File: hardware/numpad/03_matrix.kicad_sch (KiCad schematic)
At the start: 36 parts, among them SW3 RotaryEncoder_Switch

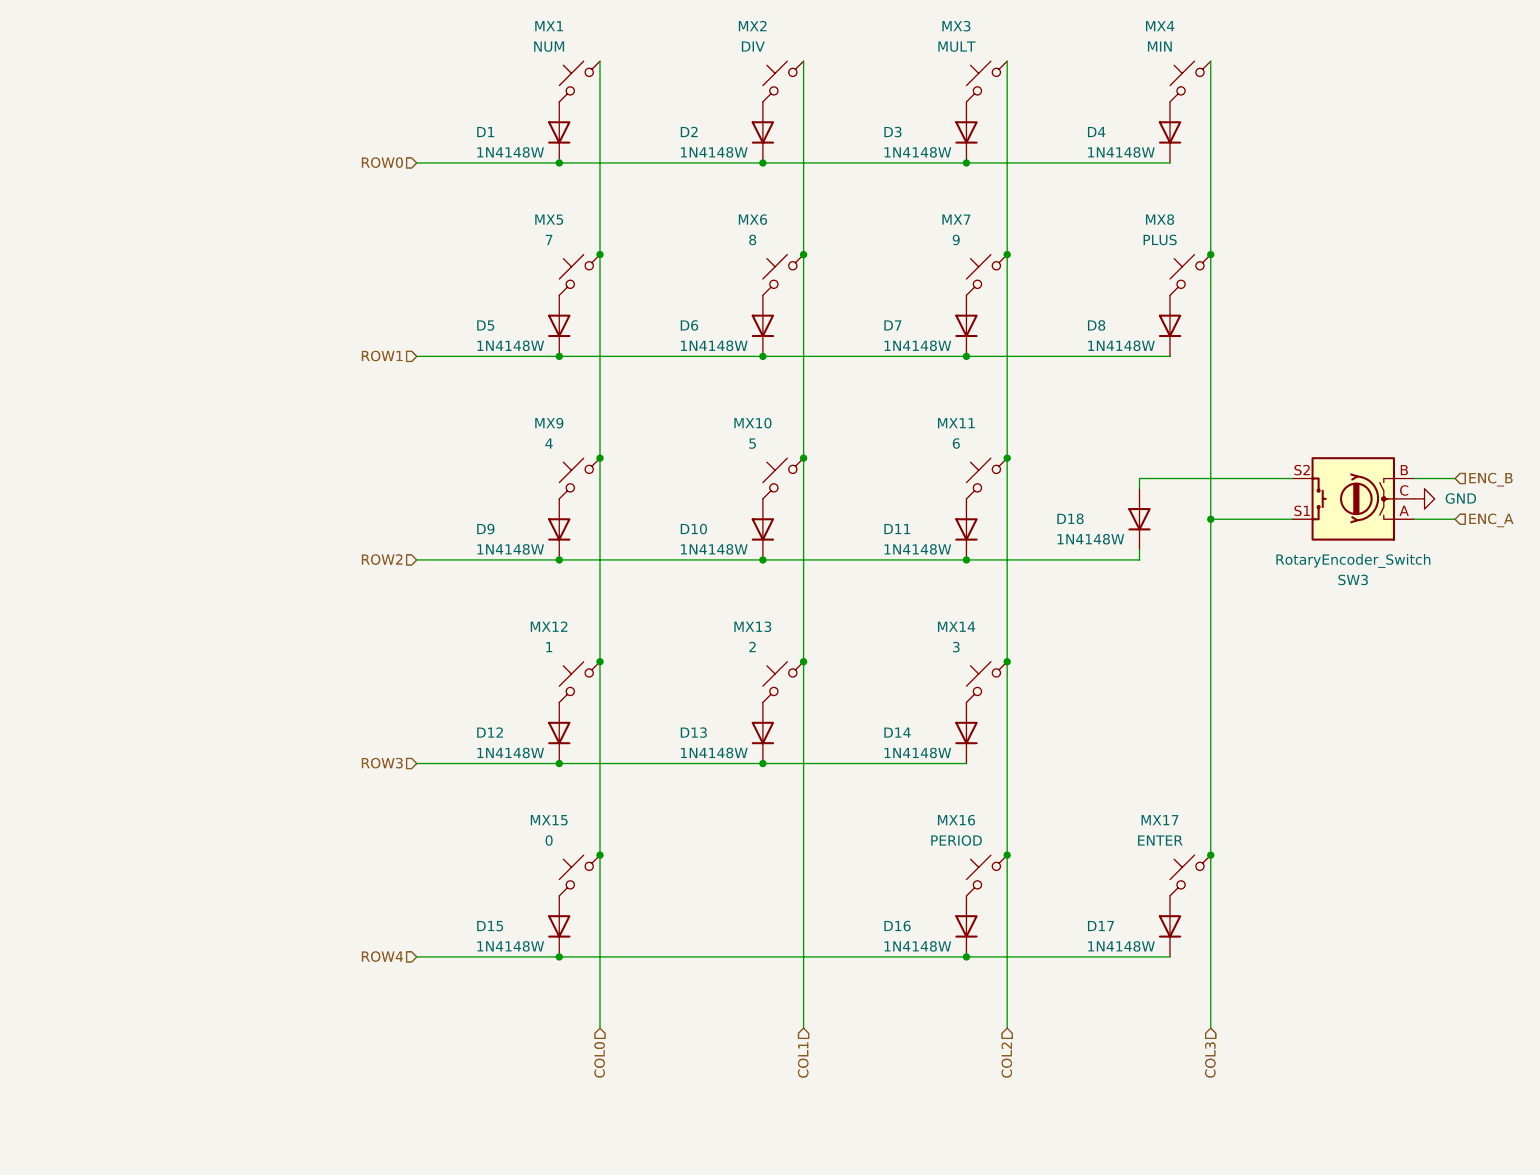
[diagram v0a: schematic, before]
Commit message: Format cleanup, titles
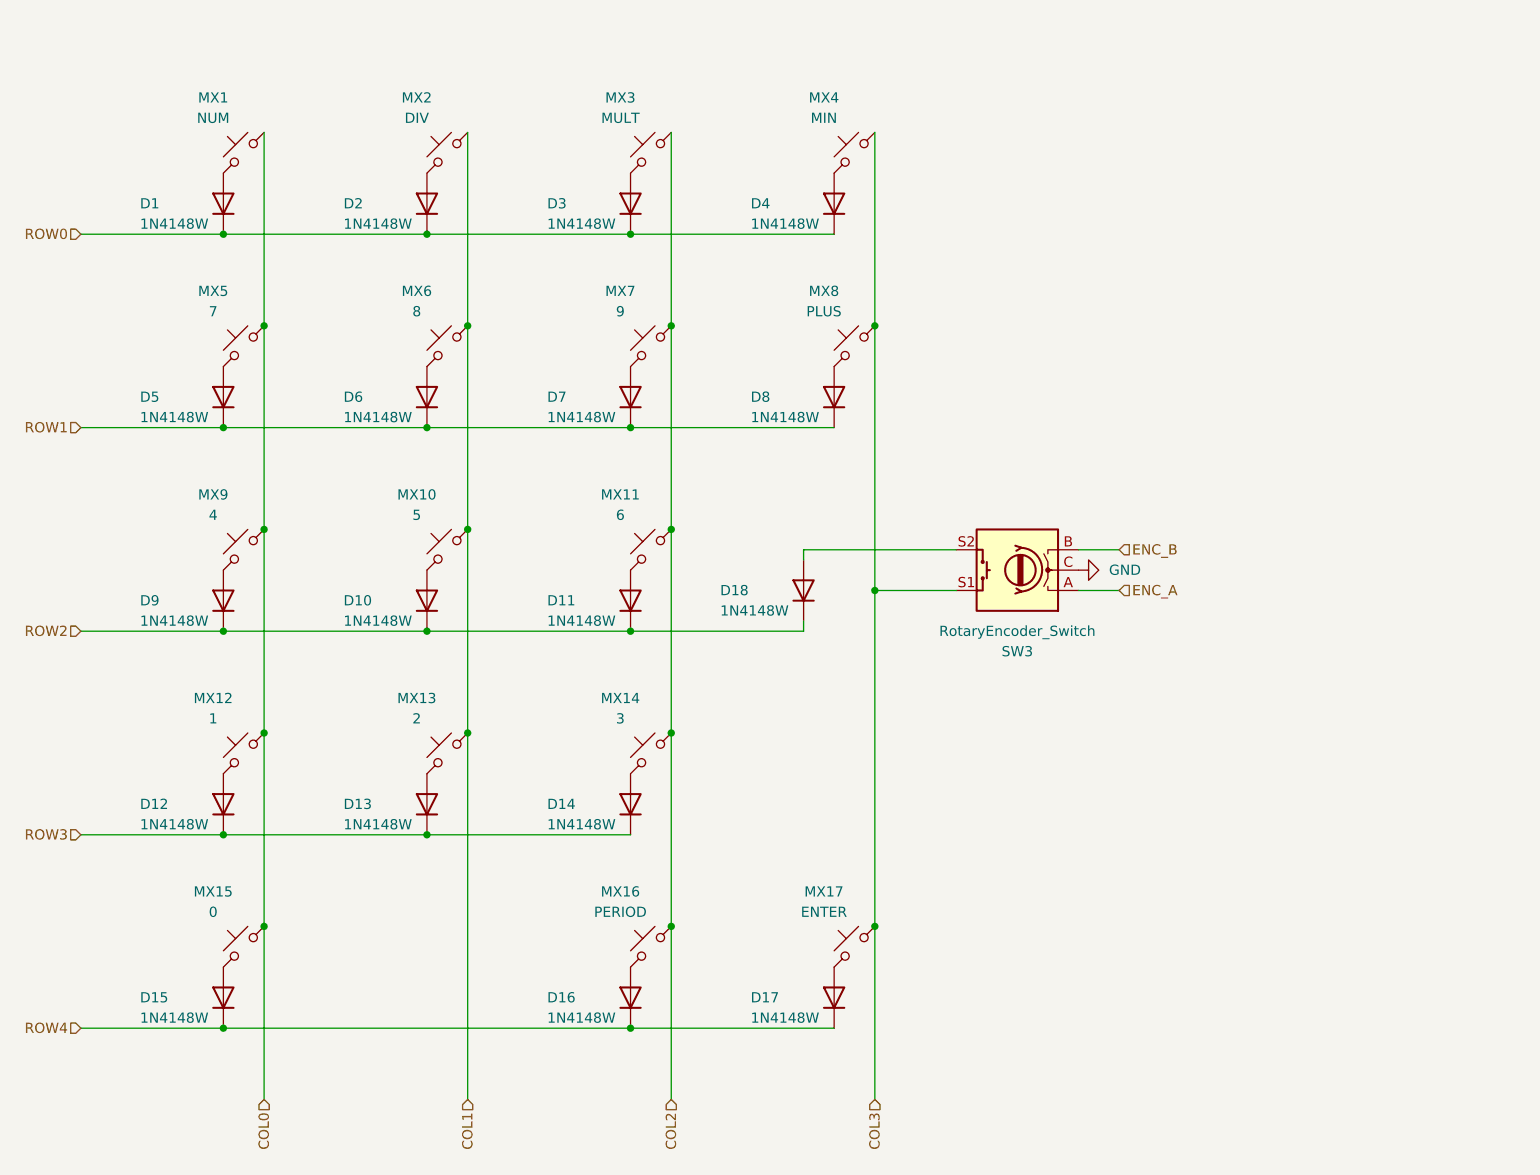
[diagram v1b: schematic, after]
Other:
- title: (none) -> Switch Matrix
- moved on the sheet: D1, D10, D11, D12, D13, D14, D15, D16, D17, D18, D2, D3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

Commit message: footprints set
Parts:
- SW3: footprint (none) -> Rotary_Encoder:RotaryEncoder_Alps_EC11E-Switch_Vertical_H20mm
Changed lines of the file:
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@@
 			)
 		)
-		(property "Footprint" ""
+		(property "Footprint" "Rotary_Encoder:RotaryEncoder_Alps_EC11E-Switch_Vertical_H20mm"
 			(at 176.53 94.234 0)
 			(hide yes)
